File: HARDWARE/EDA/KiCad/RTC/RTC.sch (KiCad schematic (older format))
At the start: 20 parts, among them J1 I2C, J2 COMPLEMENT, U1 DS1307+, U2 LM1117-ADJ, Y1 32.768

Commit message: fix trimpot footprint
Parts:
- RV1: footprint (none) -> Potentiometer_THT:Potentiometer_Bourns_3296Y_Vertical
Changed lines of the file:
@@
 F 0 "RV1" H 5380 5154 50  0000 R CNN
 F 1 "1K" H 5380 5245 50  0000 R CNN
-F 2 "" H 5450 5200 50  0001 C CNN
+F 2 "Potentiometer_THT:Potentiometer_Bourns_3296Y_Vertical" H 5450 5200 50  0001 C CNN
 F 3 "~" H 5450 5200 50  0001 C CNN
 	1    5450 5200

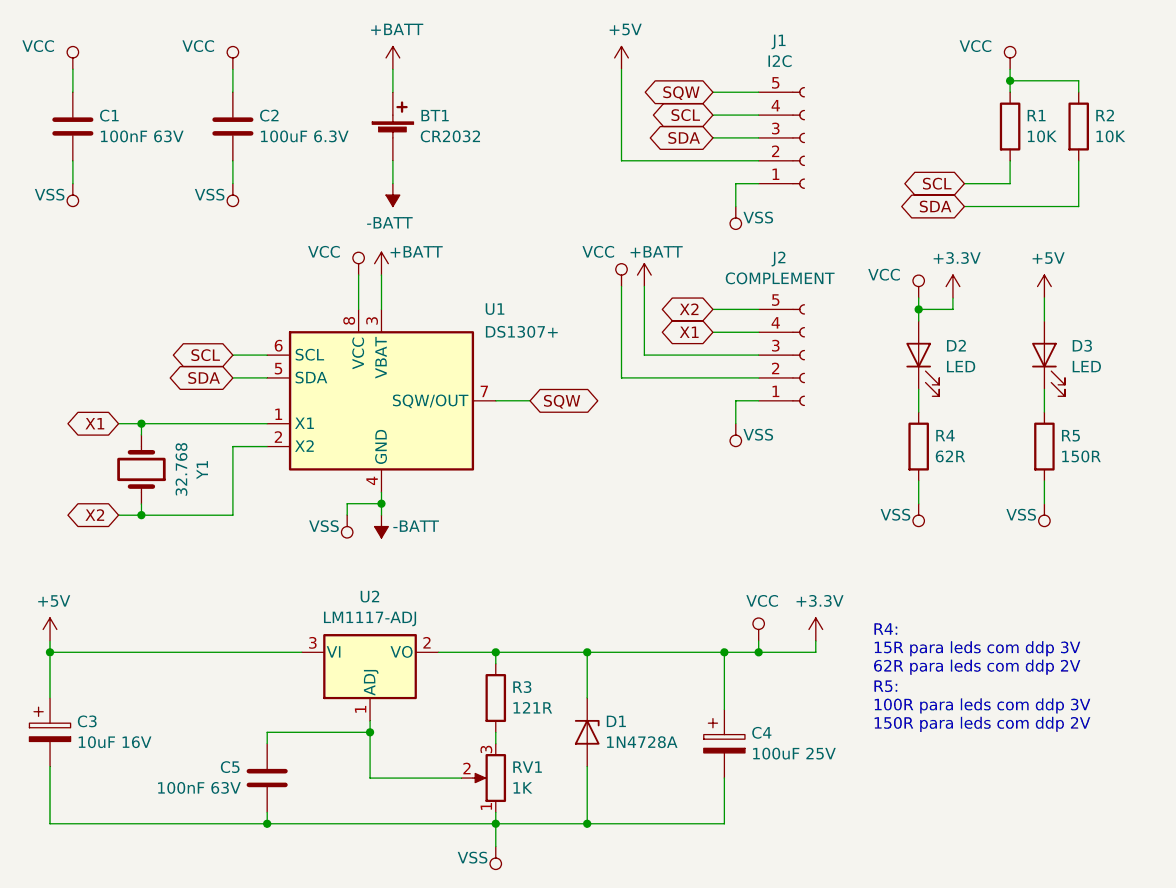
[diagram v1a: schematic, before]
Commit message: pause project
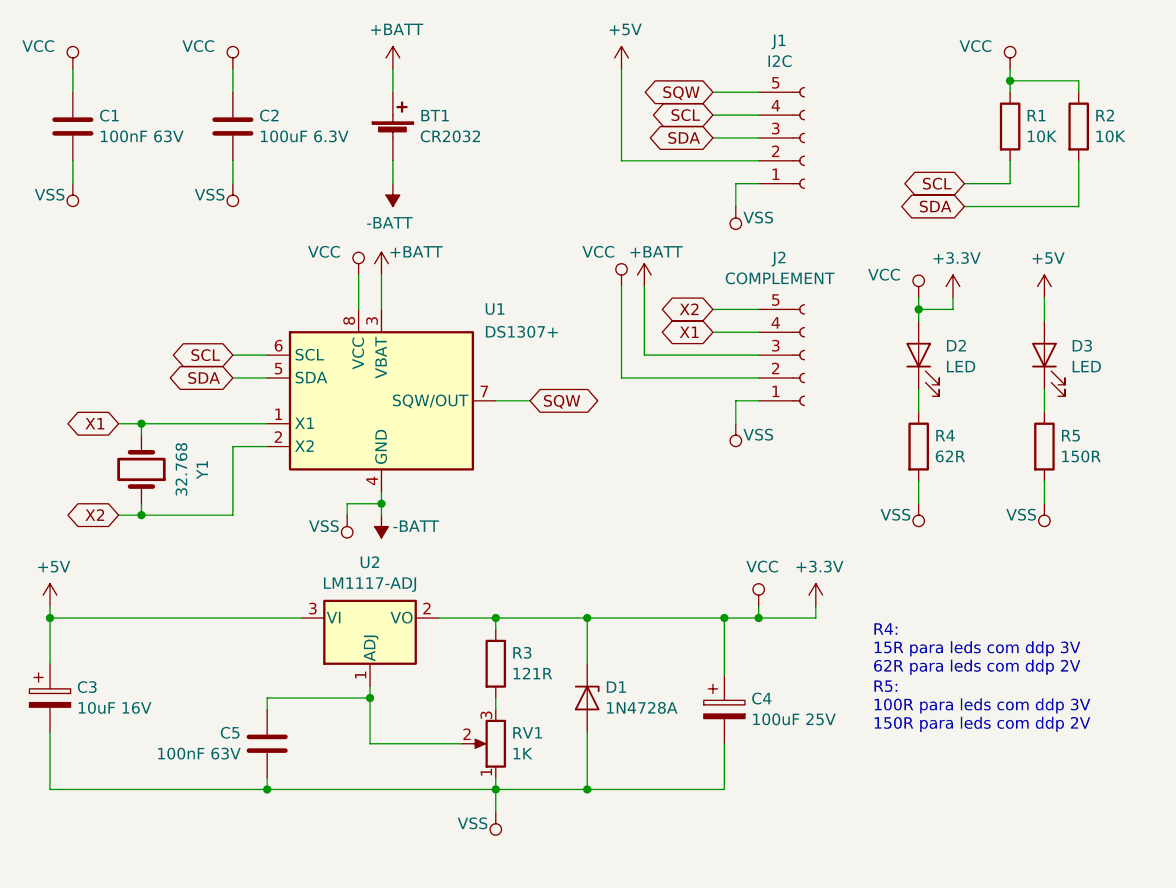
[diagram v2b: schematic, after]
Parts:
- C4: footprint Capacitor_THT:CP_Radial_D7.5mm_P2.50mm -> Capacitor_THT:CP_Radial_D5.0mm_P2.50mm
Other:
- moved on the sheet: C3, C4, C5, D1, R3, RV1, U2
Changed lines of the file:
@@
 L power:+5V #PWR017
 U 1 1 61BFACF3
-P 3500 4600
-F 0 "#PWR017" H 3500 4450 50  0001 C CNN
-F 1 "+5V" H 3515 4773 50  0000 C CNN
-F 2 "" H 3500 4600 50  0001 C CNN
-F 3 "" H 3500 4600 50  0001 C CNN
-	1    3500 4600
+P 3500 4450
+F 0 "#PWR017" H 3500 4300 50  0001 C CNN
+F 1 "+5V" H 3515 4623 50  0000 C CNN
+F 2 "" H 3500 4450 50  0001 C CNN
+F 3 "" H 3500 4450 50  0001 C CNN
+	1    3500 4450
 	1    0    0    -1
 $EndComp
@@
 L power:VSS #PWR020
 U 1 1 61C73108
-P 5450 5500
-F 0 "#PWR020" H 5450 5350 50  0001 C CNN
-F 1 "VSS" H 5550 5550 50  0000 C CNN
-F 2 "" H 5450 5500 50  0001 C CNN
-F 3 "" H 5450 5500 50  0001 C CNN
-	1    5450 5500
+P 5450 5350
+F 0 "#PWR020" H 5450 5200 50  0001 C CNN
+F 1 "VSS" H 5550 5400 50  0000 C CNN
+F 2 "" H 5450 5350 50  0001 C CNN
+F 3 "" H 5450 5350 50  0001 C CNN
+	1    5450 5350
 	-1   0    0    1
 $EndComp
@@
 L power:+3.3V #PWR019
 U 1 1 61C8D786
-P 6850 4600
-F 0 "#PWR019" H 6850 4450 50  0001 C CNN
-F 1 "+3.3V" H 6865 4773 50  0000 C CNN
-F 2 "" H 6850 4600 50  0001 C CNN
-F 3 "" H 6850 4600 50  0001 C CNN
-	1    6850 4600
-	1    0    0    -1
-$EndComp
-Wire Wire Line
-	5850 4850 5850 4650
-Wire Wire Line
-	5850 5150 5850 5400
-Wire Wire Line
-	5850 5400 5450 5400
-Wire Wire Line
-	5450 5400 5450 5500
-Wire Wire Line
-	6850 4650 6850 4600
+P 6850 4450
+F 0 "#PWR019" H 6850 4300 50  0001 C CNN
+F 1 "+3.3V" H 6865 4623 50  0000 C CNN
+F 2 "" H 6850 4450 50  0001 C CNN
+F 3 "" H 6850 4450 50  0001 C CNN
+	1    6850 4450
+	1    0    0    -1
+$EndComp
+Wire Wire Line
+	5850 4700 5850 4500
+Wire Wire Line
+	5850 5000 5850 5250
+Wire Wire Line
+	5850 5250 5450 5250
+Wire Wire Line
+	5450 5250 5450 5350
+Wire Wire Line
+	6850 4500 6850 4450
 $Comp
 L Diode:1N47xxA D1
 U 1 1 61C97F41
-P 5850 5000
-F 0 "D1" V 5804 5079 50  0000 L CNN
-F 1 "1N4728A" V 5895 5079 50  0000 L CNN
-F 2 "Diode_THT:D_DO-41_SOD81_P10.16mm_Horizontal" H 5850 4825 50  0001 C CNN
-F 3 "https://www.vishay.com/docs/85816/1n4728a.pdf" H 5850 5000 50  0001 C CNN
-	1    5850 5000
+P 5850 4850
+F 0 "D1" V 5804 4929 50  0000 L CNN
+F 1 "1N4728A" V 5895 4929 50  0000 L CNN
+F 2 "Diode_THT:D_DO-41_SOD81_P10.16mm_Horizontal" H 5850 4675 50  0001 C CNN
+F 3 "https://www.vishay.com/docs/85816/1n4728a.pdf" H 5850 4850 50  0001 C CNN
+	1    5850 4850
 	0    1    1    0
 $EndComp
@@
 L Device:CP C4
 U 1 1 61C9EDC4
-P 6450 5050
-F 0 "C4" H 6568 5096 50  0000 L CNN
-F 1 "100uF 25V" H 6568 5005 50  0000 L CNN
-F 2 "Capacitor_THT:CP_Radial_D7.5mm_P2.50mm" H 6488 4900 50  0001 C CNN
-F 3 "~" H 6450 5050 50  0001 C CNN
-	1    6450 5050
-	1    0    0    -1
-$EndComp
-Wire Wire Line
-	6450 5200 6450 5400
-Wire Wire Line
-	6450 5400 5850 5400
-Connection ~ 5850 5400
-Wire Wire Line
-	3500 5150 3500 5400
+P 6450 4900
+F 0 "C4" H 6568 4946 50  0000 L CNN
+F 1 "100uF 25V" H 6568 4855 50  0000 L CNN
+F 2 "Capacitor_THT:CP_Radial_D5.0mm_P2.50mm" H 6488 4750 50  0001 C CNN
+F 3 "~" H 6450 4900 50  0001 C CNN
+	1    6450 4900
+	1    0    0    -1
+$EndComp
+Wire Wire Line
+	6450 5050 6450 5250
+Wire Wire Line
+	6450 5250 5850 5250
+Connection ~ 5850 5250
+Wire Wire Line
+	3500 5000 3500 5250
 $Comp
 L Device:R_POT RV1
 U 1 1 61CA9B97
-P 5450 5200
-F 0 "RV1" H 5380 5154 50  0000 R CNN
-F 1 "1K" H 5380 5245 50  0000 R CNN
-F 2 "Potentiometer_THT:Potentiometer_Bourns_3296Y_Vertical" H 5450 5200 50  0001 C CNN
-F 3 "~" H 5450 5200 50  0001 C CNN
-	1    5450 5200
+P 5450 5050
+F 0 "RV1" H 5380 5004 50  0000 R CNN
+F 1 "1K" H 5380 5095 50  0000 R CNN
+F 2 "Potentiometer_THT:Potentiometer_Bourns_3296Y_Vertical" H 5450 5050 50  0001 C CNN
+F 3 "~" H 5450 5050 50  0001 C CNN
+	1    5450 5050
 	-1   0    0    1
 $EndComp
 Wire Wire Line
-	5450 5350 5450 5400
-Connection ~ 5450 5400
-Connection ~ 5850 4650
+	5450 5200 5450 5250
+Connection ~ 5450 5250
+Connection ~ 5850 4500
 $Comp
 L power:VCC #PWR018
 U 1 1 61C8DB80
-P 6600 4600
-F 0 "#PWR018" H 6600 4450 50  0001 C CNN
-F 1 "VCC" H 6617 4773 50  0000 C CNN
-F 2 "" H 6600 4600 50  0001 C CNN
-F 3 "" H 6600 4600 50  0001 C CNN
-	1    6600 4600
-	1    0    0    -1
-$EndComp
-Wire Wire Line
-	6600 4650 6850 4650
-Wire Wire Line
-	6600 4650 6600 4600
-Connection ~ 6450 4650
-Wire Wire Line
-	6450 4650 5850 4650
-Wire Wire Line
-	6450 4900 6450 4650
-Connection ~ 6600 4650
-Wire Wire Line
-	6450 4650 6600 4650
-Wire Wire Line
-	5300 5200 4900 5200
-Wire Wire Line
-	4900 5200 4900 5000
-Wire Wire Line
-	3500 4600 3500 4650
-Wire Wire Line
-	3500 4850 3500 4650
-Connection ~ 3500 4650
-Wire Wire Line
-	5200 4650 5450 4650
+P 6600 4450
+F 0 "#PWR018" H 6600 4300 50  0001 C CNN
+F 1 "VCC" H 6617 4623 50  0000 C CNN
+F 2 "" H 6600 4450 50  0001 C CNN
+F 3 "" H 6600 4450 50  0001 C CNN
+	1    6600 4450
+	1    0    0    -1
+$EndComp
+Wire Wire Line
+	6600 4500 6850 4500
+Wire Wire Line
+	6600 4500 6600 4450
+Connection ~ 6450 4500
+Wire Wire Line
+	6450 4500 5850 4500
+Wire Wire Line
+	6450 4750 6450 4500
+Connection ~ 6600 4500
+Wire Wire Line
+	6450 4500 6600 4500
+Wire Wire Line
+	5300 5050 4900 5050
+Wire Wire Line
+	4900 5050 4900 4850
+Wire Wire Line
+	3500 4450 3500 4500
+Wire Wire Line
+	3500 4700 3500 4500
+Connection ~ 3500 4500
+Wire Wire Line
+	5200 4500 5450 4500
 $Comp
 L Device:R R3
 U 1 1 61CD8F79
-P 5450 4850
-F 0 "R3" H 5520 4896 50  0000 L CNN
-F 1 "121R" H 5520 4805 50  0000 L CNN
-F 2 "Resistor_THT:R_Axial_DIN0207_L6.3mm_D2.5mm_P7.62mm_Horizontal" V 5380 4850 50  0001 C CNN
-F 3 "~" H 5450 4850 50  0001 C CNN
-	1    5450 4850
-	1    0    0    -1
-$EndComp
-Wire Wire Line
-	5450 5000 5450 5050
-Wire Wire Line
-	5450 4650 5450 4700
-Connection ~ 5450 4650
-Wire Wire Line
-	5450 4650 5850 4650
+P 5450 4700
+F 0 "R3" H 5520 4746 50  0000 L CNN
+F 1 "121R" H 5520 4655 50  0000 L CNN
+F 2 "Resistor_THT:R_Axial_DIN0207_L6.3mm_D2.5mm_P7.62mm_Horizontal" V 5380 4700 50  0001 C CNN
+F 3 "~" H 5450 4700 50  0001 C CNN
+	1    5450 4700
+	1    0    0    -1
+$EndComp
+Wire Wire Line
+	5450 4850 5450 4900
+Wire Wire Line
+	5450 4500 5450 4550
+Connection ~ 5450 4500
+Wire Wire Line
+	5450 4500 5850 4500
 $Comp
 L Device:C C5
 U 1 1 61CFECBD
-P 4450 5200
-F 0 "C5" H 4565 5246 50  0000 L CNN
-F 1 "100nF 63V" H 4565 5155 50  0000 L CNN
-F 2 "Capacitor_THT:C_Rect_L7.2mm_W2.5mm_P5.00mm_FKS2_FKP2_MKS2_MKP2" H 4488 5050 50  0001 C CNN
-F 3 "~" H 4450 5200 50  0001 C CNN
-	1    4450 5200
+P 4450 5050
+F 0 "C5" H 4565 5096 50  0000 L CNN
+F 1 "100nF 63V" H 4565 5005 50  0000 L CNN
+F 2 "Capacitor_THT:C_Rect_L7.2mm_W2.5mm_P5.00mm_FKS2_FKP2_MKS2_MKP2" H 4488 4900 50  0001 C CNN
+F 3 "~" H 4450 5050 50  0001 C CNN
+	1    4450 5050
 	-1   0    0    -1
 $EndComp
 Wire Wire Line
-	4450 5350 4450 5400
-Wire Wire Line
-	4450 5400 5450 5400
-Wire Wire Line
-	4450 5400 3500 5400
-Connection ~ 4450 5400
-Wire Wire Line
-	3500 4650 4600 4650
-Wire Wire Line
-	4450 5050 4450 5000
-Wire Wire Line
-	4450 5000 4900 5000
-Connection ~ 4900 5000
-Wire Wire Line
-	4900 5000 4900 4950
+	4450 5200 4450 5250
+Wire Wire Line
+	4450 5250 5450 5250
+Wire Wire Line
+	4450 5250 3500 5250
+Connection ~ 4450 5250
+Wire Wire Line
+	3500 4500 4600 4500
+Wire Wire Line
+	4450 4900 4450 4850
+Wire Wire Line
+	4450 4850 4900 4850
+Connection ~ 4900 4850
+Wire Wire Line
+	4900 4850 4900 4800
 $Comp
 L Regulator_Linear:LM1117-ADJ U2
 U 1 1 61D2766B
-P 4900 4650
-F 0 "U2" H 4900 4892 50  0000 C CNN
-F 1 "LM1117-ADJ" H 4900 4801 50  0000 C CNN
-F 2 "Package_TO_SOT_THT:TO-220-3_Vertical" H 4900 4650 50  0001 C CNN
-F 3 "http://www.ti.com/lit/ds/symlink/lm1117.pdf" H 4900 4650 50  0001 C CNN
-	1    4900 4650
+P 4900 4500
+F 0 "U2" H 4900 4742 50  0000 C CNN
+F 1 "LM1117-ADJ" H 4900 4651 50  0000 C CNN
+F 2 "Package_TO_SOT_THT:TO-220-3_Vertical" H 4900 4500 50  0001 C CNN
+F 3 "http://www.ti.com/lit/ds/symlink/lm1117.pdf" H 4900 4500 50  0001 C CNN
+	1    4900 4500
 	1    0    0    -1
 $EndComp
@@
 L Device:CP C3
 U 1 1 61CA46D0
-P 3500 5000
-F 0 "C3" H 3618 5046 50  0000 L CNN
-F 1 "10uF 16V" H 3618 4955 50  0000 L CNN
-F 2 "Capacitor_THT:CP_Radial_D5.0mm_P2.00mm" H 3538 4850 50  0001 C CNN
-F 3 "~" H 3500 5000 50  0001 C CNN
-	1    3500 5000
-	1    0    0    -1
-$EndComp
+P 3500 4850
+F 0 "C3" H 3618 4896 50  0000 L CNN
+F 1 "10uF 16V" H 3618 4805 50  0000 L CNN
+F 2 "Capacitor_THT:CP_Radial_D5.0mm_P2.00mm" H 3538 4700 50  0001 C CNN
+F 3 "~" H 3500 4850 50  0001 C CNN
+	1    3500 4850
+	1    0    0    -1
+$EndComp
